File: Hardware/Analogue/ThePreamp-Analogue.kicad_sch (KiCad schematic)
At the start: 31 parts, among them IC1 ULN2803CDWR, J1 To preamp, J2 From preamp, J3 Digital In, J4 Digital Pass Through, J5 Power In, J6 Power Out, J7 ADS1115, J8 Replace, J9 Replace, K1 Input 1, K2 Input 2, K3 Input 3, K4 Input 4, K5 Output Mute, U1 MCP23008-E_SO

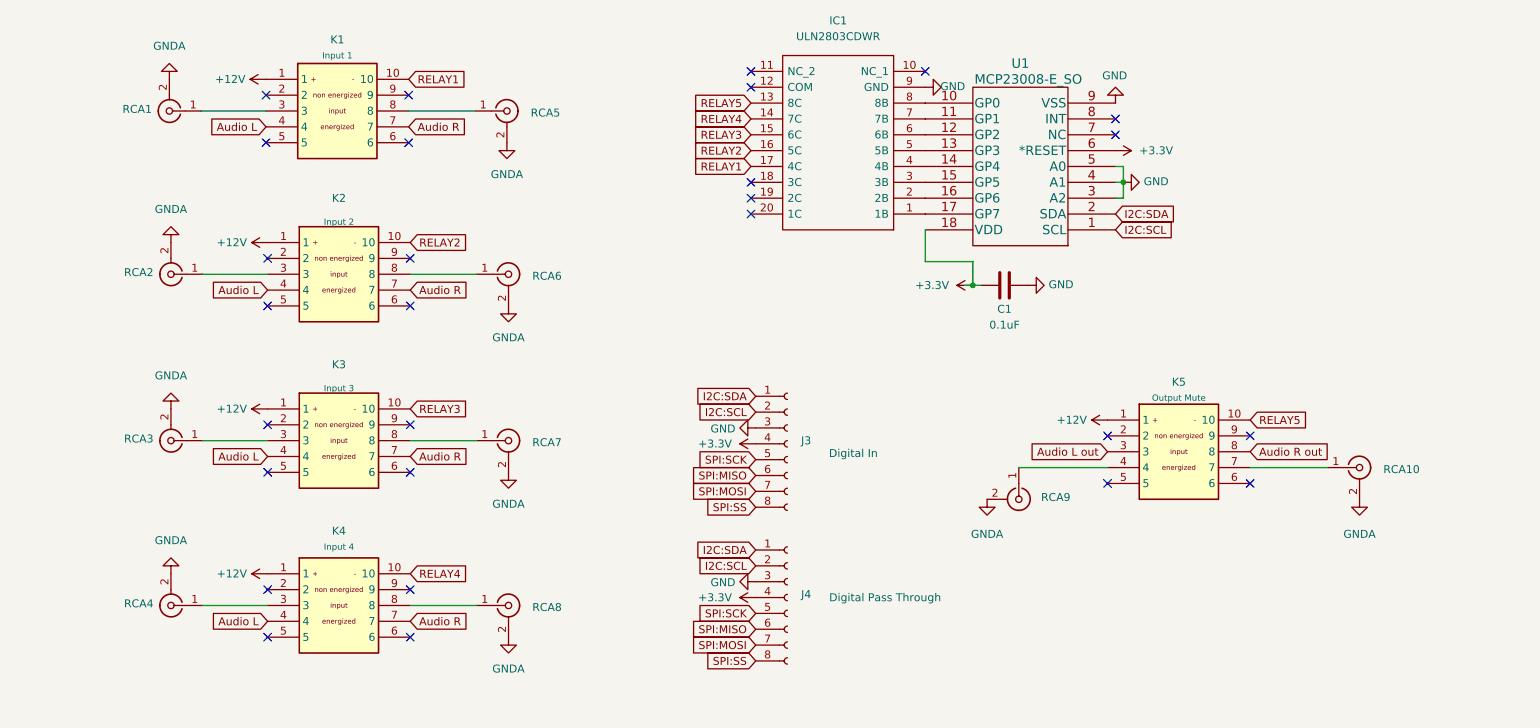
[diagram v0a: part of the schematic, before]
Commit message: pcb redesign
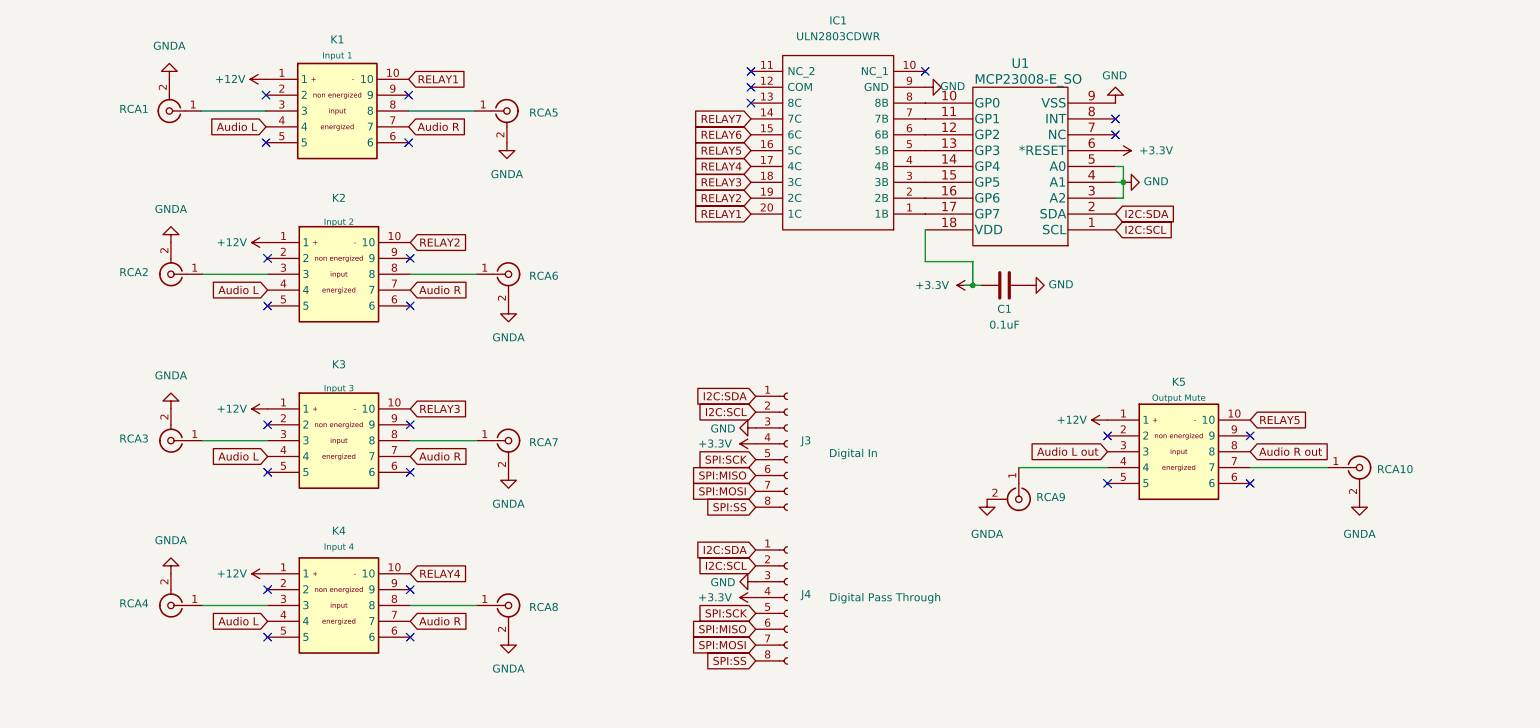
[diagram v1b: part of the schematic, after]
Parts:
- IC1: footprint SOIC127P1030X265-20N -> ULN2803:SOIC127P1030X265-20N
- RCA1, RCA2, RCA5, RCA6: footprint Connector_Audio:RCA Connector ALI -> RCA ALI:RCA Connector ALI; symbol Connector:RCA_Connector_ALI -> RCA ALI:RCA_Connector_ALI
- RCA10, RCA3, RCA4, RCA7, RCA8, RCA9: symbol Connector:RCA_Connector_ALI -> RCA ALI:RCA_Connector_ALI
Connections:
- net RELAY1: now also IC1.20 (1C); no longer IC1.17 (4C)
- net RELAY2: now also IC1.19 (2C); no longer IC1.16 (5C)
- net RELAY3: now also IC1.18 (3C); no longer IC1.15 (6C)
- net RELAY4: now also IC1.17 (4C); no longer IC1.14 (7C)
- net RELAY5: now also IC1.16 (5C); no longer IC1.13 (8C)
- new net RELAY6: IC1.15 (6C)
- new net RELAY7: IC1.14 (7C)
- no-connect marks 31 -> 29
